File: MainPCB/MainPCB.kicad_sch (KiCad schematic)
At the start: 0 parts

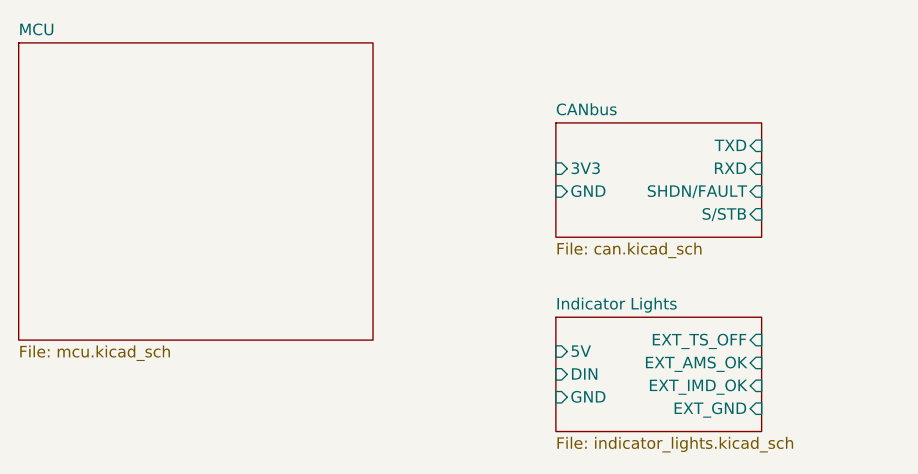
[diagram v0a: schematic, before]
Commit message: MCU design + global power supplies
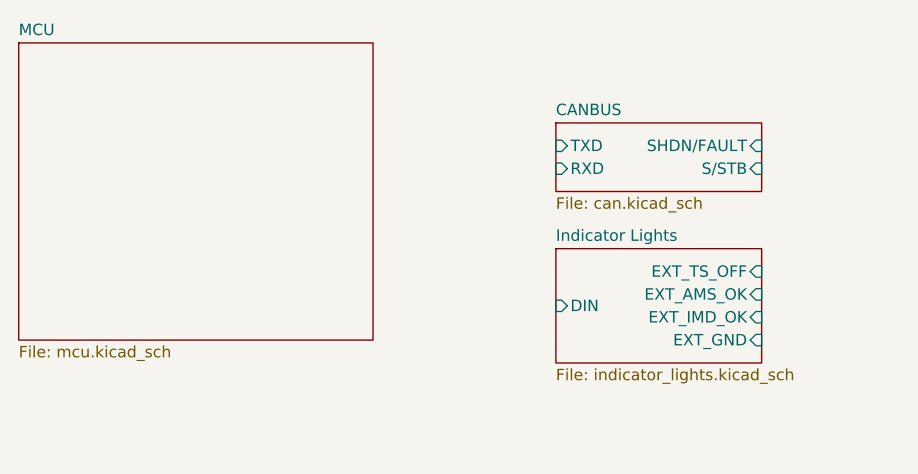
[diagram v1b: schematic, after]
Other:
- sheet CANbus renamed CANBUS
- sheet CANBUS ports: added none; removed 3V3, GND
- sheet Indicator Lights ports: added none; removed 5V, GND
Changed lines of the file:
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@@
 	(sheet
 		(at 86.36 33.02)
-		(size 22.86 12.7)
+		(size 22.86 7.62)
 		(exclude_from_sim no)
 		(in_bom yes)
@@
 			(color 0 0 0 0.0000)
 		)
-		(property "Sheetname" "CANbus"
+		(property "Sheetname" "CANBUS"
 			(at 86.36 32.3084 0)
 			(effects
@@
 		)
 		(property "Sheetfile" "can.kicad_sch"
-			(at 86.36 46.3046 0)
+			(at 86.36 41.2246 0)
 			(effects
 				(font
@@
 		)
 		(pin "S{slash}STB" input
-			(at 109.22 43.18 0)
+			(at 109.22 38.1 0)
 			(effects
 				(font
@@
 		)
 		(pin "TXD" input
-			(at 109.22 35.56 0)
+			(at 86.36 35.56 180)
 			(effects
 				(font
 					(size 1.27 1.27)
 				)
-				(justify right)
+				(justify left)
 			)
 		)
 		(pin "RXD" input
-			(at 109.22 38.1 0)
-			(effects
-				(font
-					(size 1.27 1.27)
-				)
-				(justify right)
-			)
-		)
-		(pin "GND" input
-			(at 86.36 40.64 180)
+			(at 86.36 38.1 180)
 			(effects
 				(font
@@
 		)
 		(pin "SHDN{slash}FAULT" input
-			(at 109.22 40.64 0)
+			(at 109.22 35.56 0)
 			(effects
 				(font
@@
 				)
 				(justify right)
-			)
-		)
-		(pin "3V3" input
-			(at 86.36 38.1 180)
-			(effects
-				(font
-					(size 1.27 1.27)
-				)
-				(justify left)
 			)
 		)
@@
 	)
 	(sheet
-		(at 86.36 54.61)
+		(at 86.36 46.99)
 		(size 22.86 12.7)
 		(exclude_from_sim no)
@@
 		)
 		(property "Sheetname" "Indicator Lights"
-			(at 86.36 53.8984 0)
+			(at 86.36 46.2784 0)
 			(effects
 				(font
@@
 		)
 		(property "Sheetfile" "indicator_lights.kicad_sch"
-			(at 86.36 67.8946 0)
+			(at 86.36 60.2746 0)
 			(effects
 				(font
@@
 			)
 		)
-		(pin "5V" input
-			(at 86.36 58.42 180)
-			(effects
-				(font
-					(size 1.27 1.27)
-				)
-				(justify left)
-			)
-		)
 		(pin "DIN" input
-			(at 86.36 60.96 180)
-			(effects
-				(font
-					(size 1.27 1.27)
-				)
-				(justify left)
-			)
-		)
-		(pin "GND" input
-			(at 86.36 63.5 180)
+			(at 86.36 53.34 180)
 			(effects
 				(font
@@
 		)
 		(pin "EXT_TS_OFF" input
-			(at 109.22 57.15 0)
+			(at 109.22 49.53 0)
 			(effects
 				(font
@@
 		)
 		(pin "EXT_AMS_OK" input
-			(at 109.22 59.69 0)
+			(at 109.22 52.07 0)
 			(effects
 				(font
@@
 		)
 		(pin "EXT_IMD_OK" input
-			(at 109.22 62.23 0)
+			(at 109.22 54.61 0)
 			(effects
 				(font
@@
 		)
 		(pin "EXT_GND" input
-			(at 109.22 64.77 0)
+			(at 109.22 57.15 0)
 			(effects
 				(font
